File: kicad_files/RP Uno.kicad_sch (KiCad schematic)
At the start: 58 parts, among them J1 USB_B, J2 Conn_01x08, J3 Conn_01x06, J4 Conn_01x10, J5 Conn_01x08, J6 Barrel_Jack_Switch, J7 ICSP, J8 SWD, Q1 FDN340P, Q2 FDN340P, SW1 1-1437565-7, SW2 BOOTSEL, U1 RP2040, U2 74LVC1G125, U3 AP2112K-3.3, U4 W25Q32JVSS, U5 NCP1117-5.0_SOT223, Y1 12MHz

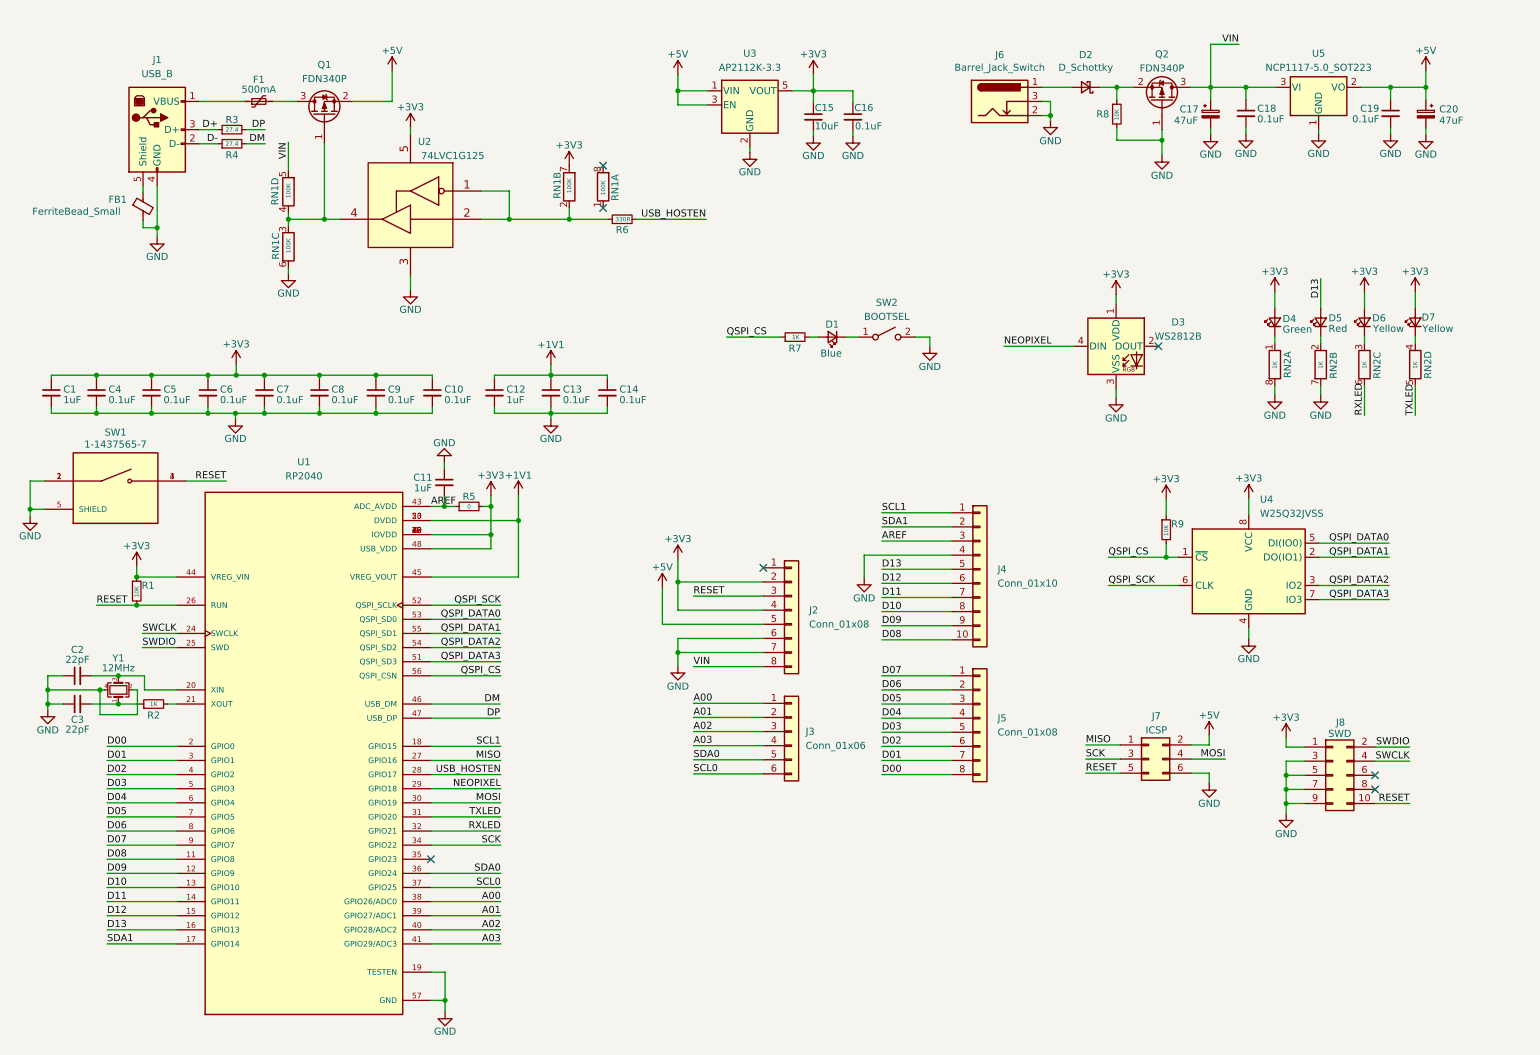
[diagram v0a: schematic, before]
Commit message: Partial Rev 2 updates
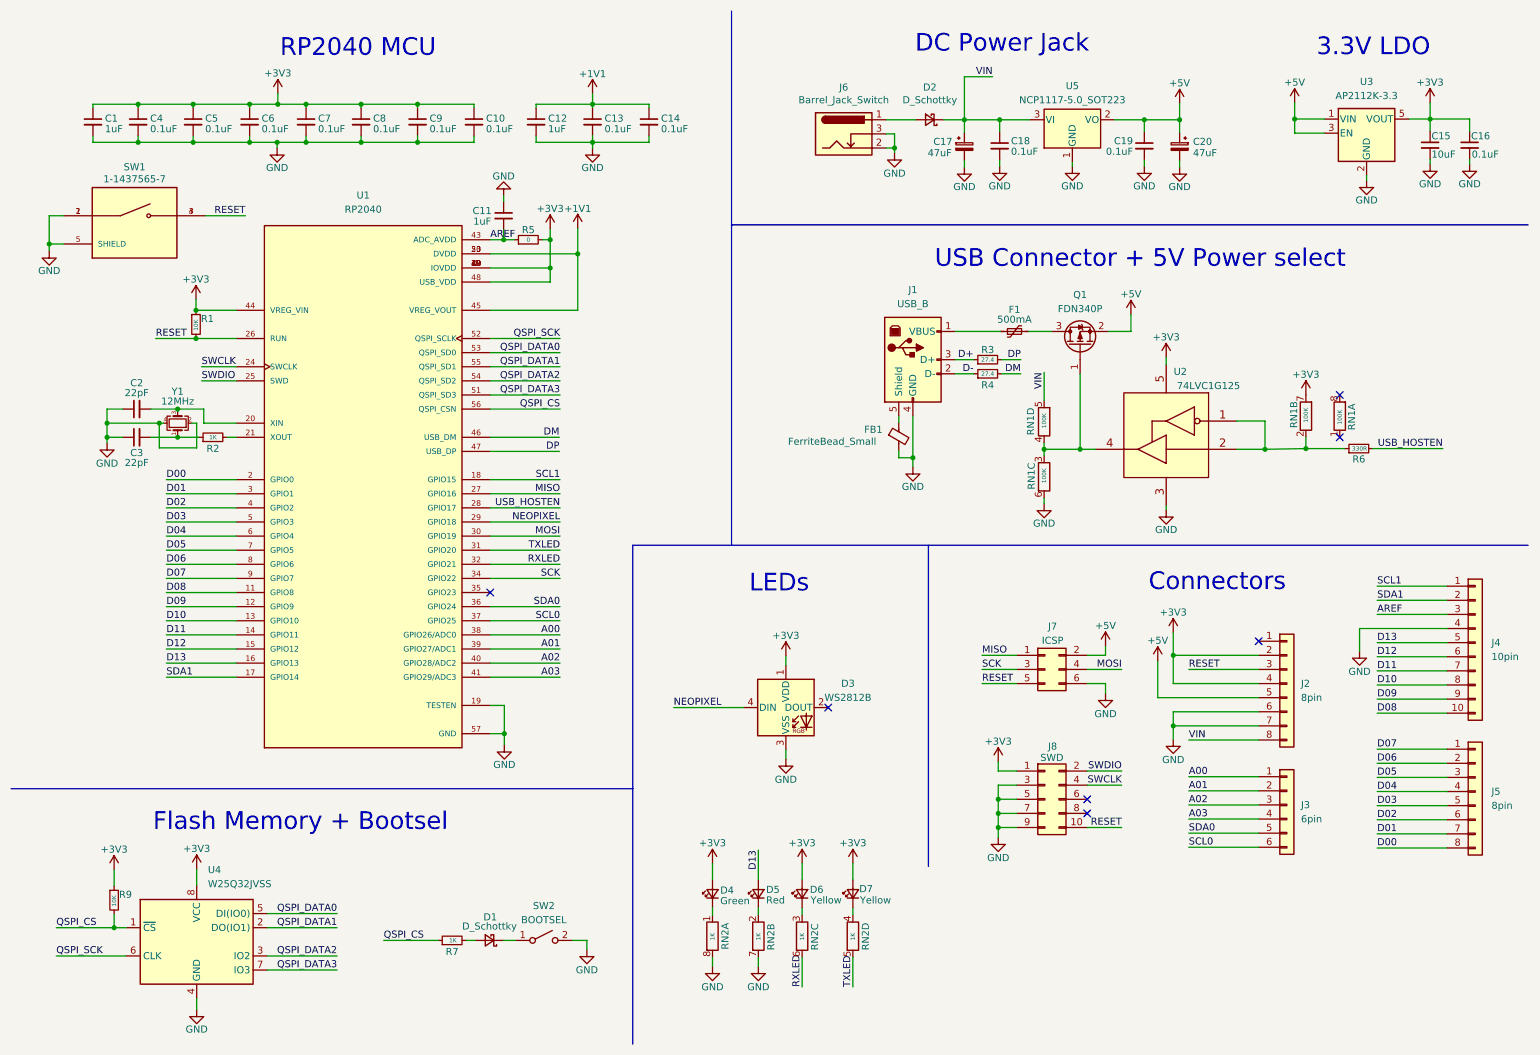
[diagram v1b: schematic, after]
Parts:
- removed D1: Blue, LED_SMD:LED_0603_1608Metric, symbol Device:LED_Small
- removed Q2: FDN340P, Package_TO_SOT_SMD:SOT-23, symbol Transistor_FET:FDN340P
- removed R8: 10K, Resistor_SMD:R_0603_1608Metric, symbol Device:R_Small
- added D1: D_Schottky, Diode_SMD:D_SOD-323, symbol Device:D_Schottky_Small
- J2, J5: value Conn_01x08 -> 8pin
- J3: value Conn_01x06 -> 6pin
- J4: value Conn_01x10 -> 10pin
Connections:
- net VIN: now also D2.1 (K)
- net at SW2.1 (A): now also D1.1 (K)
- net at R7.2: now also D1.2 (A)
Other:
- note added: "3.3V LDO"
- note added: "Connectors"
- note added: "DC Power Jack"
- note added: "Flash Memory + Bootsel"
- note added: "LEDs"
- note added: "RP2040 MCU"
- note added: "USB Connector + 5V Power select"
- moved on the sheet: C1, C10, C11, C12, C13, C14, C15, C16, C17, C18, C19, C2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
